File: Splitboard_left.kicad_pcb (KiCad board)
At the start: 2 copper layers, 124.1 x 95.1 mm, 63 parts, among them J1 USB_C_Receptacle_USB2.0, J2 TRRS, U1 ATmega32U4-AU, Y1 16MHz

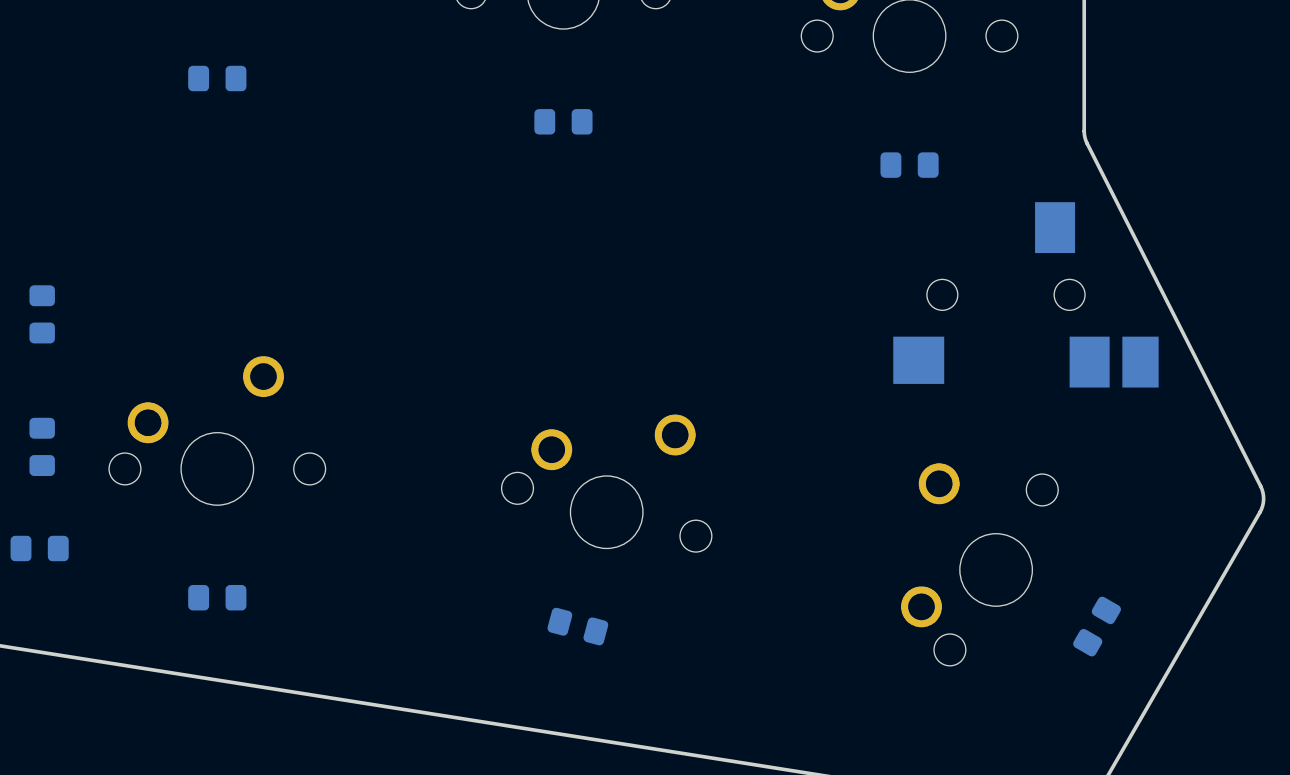
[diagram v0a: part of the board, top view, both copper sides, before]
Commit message: save
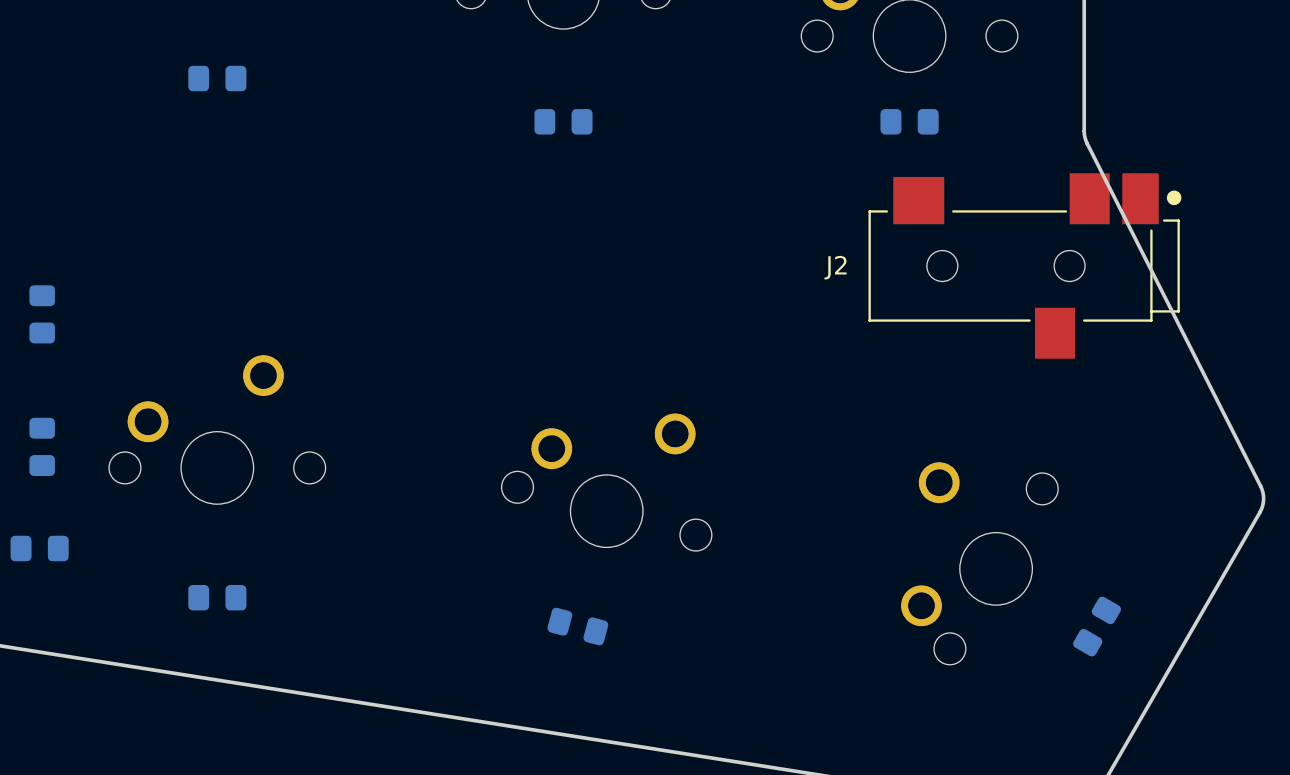
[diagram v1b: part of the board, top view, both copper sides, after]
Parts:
- J2: moved to F.Cu
- moved D52 2.38 mm to (176.9, 89.6)
- moved J2 1.59 mm to (182.5, 97.6)
- moved KC_53 0.06 mm to (181.7, 114.2)
- moved KC_43 0.06 mm to (160.3, 111.1)
- moved KC_33 0.06 mm to (138.8, 108.7)
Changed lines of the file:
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@@
   )
   (module MX_Only:MXOnly-1U-NoLED (layer F.Cu)
-    (at 181.673257 114.298749 60)
+    (at 181.673257 114.239952 60)
     (fp_text reference KC_53 (at 0 3.175 60) (layer Dwgs.User)
       (effects (font (size 1 1) (thickness 0.15)))
@@
   )
   (module MX_Only:MXOnly-1U-NoLED (layer F.Cu)
-    (at 160.253266 111.123749 345)
+    (at 160.253266 111.06662 345)
     (fp_text reference KC_43 (at 0 3.175 165) (layer Dwgs.User)
       (effects (font (size 1 1) (thickness 0.15)))
@@
   )
   (module MX_Only:MXOnly-1U-NoLED (layer F.Cu)
-    (at 138.833275 108.742499)
+    (at 138.833275 108.686621)
     (fp_text reference KC_33 (at 0 3.175) (layer Dwgs.User)
       (effects (font (size 1 1) (thickness 0.15)))
@@
     (pad "" np_thru_hole circle (at 5.08 0 48.0996) (size 1.75 1.75) (drill 1.75) (layers *.Cu *.Mask))
   )
-  (module SJ-43514-SMT:CUI_SJ-43514-SMT (layer B.Cu)
-    (at 182.46659 99.166625 180)
-    (fp_text reference J2 (at 9.519996 0) (layer B.SilkS)
-      (effects (font (size 1.004591 1.004591) (thickness 0.15)) (justify mirror))
-    )
-    (fp_text value TRRS (at 0.91336 -6.392105) (layer B.Fab)
-      (effects (font (size 1.003724 1.003724) (thickness 0.015)) (justify mirror))
-    )
-    (fp_line (start -9.5 -2.75) (end -9.5 2.75) (layer B.CrtYd) (width 0.05))
-    (fp_line (start -8.5 -2.75) (end -9.5 -2.75) (layer B.CrtYd) (width 0.05))
-    (fp_line (start -8.5 -5.5) (end -8.5 -2.75) (layer B.CrtYd) (width 0.05))
-    (fp_line (start -3 -5.5) (end -8.5 -5.5) (layer B.CrtYd) (width 0.05))
-    (fp_line (start -3 -3.25) (end -3 -5.5) (layer B.CrtYd) (width 0.05))
-    (fp_line (start 3.25 -3.25) (end -3 -3.25) (layer B.CrtYd) (width 0.05))
-    (fp_line (start 3.25 -5.5) (end 3.25 -3.25) (layer B.CrtYd) (width 0.05))
-    (fp_line (start 6.75 -5.5) (end 3.25 -5.5) (layer B.CrtYd) (width 0.05))
-    (fp_line (start 6.75 -3.25) (end 6.75 -5.5) (layer B.CrtYd) (width 0.05))
-    (fp_line (start 8 -3.25) (end 6.75 -3.25) (layer B.CrtYd) (width 0.05))
-    (fp_line (start 8 3.25) (end 8 -3.25) (layer B.CrtYd) (width 0.05))
-    (fp_line (start -1.1 3.25) (end 8 3.25) (layer B.CrtYd) (width 0.05))
-    (fp_line (start -1.1 5.35) (end -1.1 3.25) (layer B.CrtYd) (width 0.05))
-    (fp_line (start -3.8 5.35) (end -1.1 5.35) (layer B.CrtYd) (width 0.05))
-    (fp_line (start -3.8 3.25) (end -3.8 5.35) (layer B.CrtYd) (width 0.05))
-    (fp_line (start -8 3.25) (end -3.8 3.25) (layer B.CrtYd) (width 0.05))
-    (fp_line (start -8 2.75) (end -8 3.25) (layer B.CrtYd) (width 0.05))
-    (fp_line (start -9.5 2.75) (end -8 2.75) (layer B.CrtYd) (width 0.05))
-    (fp_line (start 7.75 3) (end 7.75 -3) (layer B.SilkS) (width 0.127))
-    (fp_circle (center -9 -3.75) (end -8.8 -3.75) (layer B.SilkS) (width 0.4))
-    (fp_line (start 7.75 3) (end -1.05 3) (layer B.SilkS) (width 0.127))
-    (fp_line (start 6.8 -3) (end 7.75 -3) (layer B.SilkS) (width 0.127))
-    (fp_line (start -3.05 -3) (end 3.15 -3) (layer B.SilkS) (width 0.127))
-    (fp_line (start -9.25 -2.5) (end -8.45 -2.5) (layer B.SilkS) (width 0.127))
-    (fp_line (start -9.25 2.5) (end -9.25 -2.5) (layer B.SilkS) (width 0.127))
-    (fp_line (start -7.75 2.5) (end -9.25 2.5) (layer B.SilkS) (width 0.127))
-    (fp_line (start -7.75 2.5) (end -7.75 -1.95) (layer B.SilkS) (width 0.127))
-    (fp_line (start -7.75 3) (end -7.75 2.5) (layer B.SilkS) (width 0.127))
-    (fp_line (start -4.05 3) (end -7.75 3) (layer B.SilkS) (width 0.127))
-    (fp_line (start -9.25 -2.5) (end -7.75 -2.5) (layer B.Fab) (width 0.127))
-    (fp_line (start -9.25 2.5) (end -9.25 -2.5) (layer B.Fab) (width 0.127))
-    (fp_line (start -7.75 2.5) (end -9.25 2.5) (layer B.Fab) (width 0.127))
-    (fp_line (start 7.75 3) (end -7.75 3) (layer B.Fab) (width 0.127))
-    (fp_line (start 7.75 -3) (end 7.75 3) (layer B.Fab) (width 0.127))
-    (fp_line (start -7.75 -3) (end 7.75 -3) (layer B.Fab) (width 0.127))
-    (fp_line (start -7.75 -2.5) (end -7.75 -3) (layer B.Fab) (width 0.127))
-    (fp_line (start -7.75 2.5) (end -7.75 -2.5) (layer B.Fab) (width 0.127))
-    (fp_line (start -7.75 3) (end -7.75 2.5) (layer B.Fab) (width 0.127))
+  (module SJ-43514-SMT:CUI_SJ-43514-SMT (layer F.Cu)
+    (at 182.46659 97.579959 180)
+    (fp_text reference J2 (at 9.519996 0) (layer F.SilkS)
+      (effects (font (size 1.004591 1.004591) (thickness 0.15)))
+    )
+    (fp_text value TRRS (at 0.91336 6.392105) (layer F.Fab)
+      (effects (font (size 1.003724 1.003724) (thickness 0.015)))
+    )
+    (fp_line (start -9.5 2.75) (end -9.5 -2.75) (layer F.CrtYd) (width 0.05))
+    (fp_line (start -8.5 2.75) (end -9.5 2.75) (layer F.CrtYd) (width 0.05))
+    (fp_line (start -8.5 5.5) (end -8.5 2.75) (layer F.CrtYd) (width 0.05))
+    (fp_line (start -3 5.5) (end -8.5 5.5) (layer F.CrtYd) (width 0.05))
+    (fp_line (start -3 3.25) (end -3 5.5) (layer F.CrtYd) (width 0.05))
+    (fp_line (start 3.25 3.25) (end -3 3.25) (layer F.CrtYd) (width 0.05))
+    (fp_line (start 3.25 5.5) (end 3.25 3.25) (layer F.CrtYd) (width 0.05))
+    (fp_line (start 6.75 5.5) (end 3.25 5.5) (layer F.CrtYd) (width 0.05))
+    (fp_line (start 6.75 3.25) (end 6.75 5.5) (layer F.CrtYd) (width 0.05))
+    (fp_line (start 8 3.25) (end 6.75 3.25) (layer F.CrtYd) (width 0.05))
+    (fp_line (start 8 -3.25) (end 8 3.25) (layer F.CrtYd) (width 0.05))
+    (fp_line (start -1.1 -3.25) (end 8 -3.25) (layer F.CrtYd) (width 0.05))
+    (fp_line (start -1.1 -5.35) (end -1.1 -3.25) (layer F.CrtYd) (width 0.05))
+    (fp_line (start -3.8 -5.35) (end -1.1 -5.35) (layer F.CrtYd) (width 0.05))
+    (fp_line (start -3.8 -3.25) (end -3.8 -5.35) (layer F.CrtYd) (width 0.05))
+    (fp_line (start -8 -3.25) (end -3.8 -3.25) (layer F.CrtYd) (width 0.05))
+    (fp_line (start -8 -2.75) (end -8 -3.25) (layer F.CrtYd) (width 0.05))
+    (fp_line (start -9.5 -2.75) (end -8 -2.75) (layer F.CrtYd) (width 0.05))
+    (fp_line (start 7.75 -3) (end 7.75 3) (layer F.SilkS) (width 0.127))
+    (fp_circle (center -9 3.75) (end -8.8 3.75) (layer F.SilkS) (width 0.4))
+    (fp_line (start 7.75 -3) (end -1.05 -3) (layer F.SilkS) (width 0.127))
+    (fp_line (start 6.8 3) (end 7.75 3) (layer F.SilkS) (width 0.127))
+    (fp_line (start -3.05 3) (end 3.15 3) (layer F.SilkS) (width 0.127))
+    (fp_line (start -9.25 2.5) (end -8.45 2.5) (layer F.SilkS) (width 0.127))
+    (fp_line (start -9.25 -2.5) (end -9.25 2.5) (layer F.SilkS) (width 0.127))
+    (fp_line (start -7.75 -2.5) (end -9.25 -2.5) (layer F.SilkS) (width 0.127))
+    (fp_line (start -7.75 -2.5) (end -7.75 1.95) (layer F.SilkS) (width 0.127))
+    (fp_line (start -7.75 -3) (end -7.75 -2.5) (layer F.SilkS) (width 0.127))
+    (fp_line (start -4.05 -3) (end -7.75 -3) (layer F.SilkS) (width 0.127))
+    (fp_line (start -9.25 2.5) (end -7.75 2.5) (layer F.Fab) (width 0.127))
+    (fp_line (start -9.25 -2.5) (end -9.25 2.5) (layer F.Fab) (width 0.127))
+    (fp_line (start -7.75 -2.5) (end -9.25 -2.5) (layer F.Fab) (width 0.127))
+    (fp_line (start 7.75 -3) (end -7.75 -3) (layer F.Fab) (width 0.127))
+    (fp_line (start 7.75 3) (end 7.75 -3) (layer F.Fab) (width 0.127))
+    (fp_line (start -7.75 3) (end 7.75 3) (layer F.Fab) (width 0.127))
+    (fp_line (start -7.75 2.5) (end -7.75 3) (layer F.Fab) (width 0.127))
+    (fp_line (start -7.75 -2.5) (end -7.75 2.5) (layer F.Fab) (width 0.127))
+    (fp_line (start -7.75 -3) (end -7.75 -2.5) (layer F.Fab) (width 0.127))
     (pad None np_thru_hole circle (at 3.75 0 180) (size 1.7 1.7) (drill 1.7) (layers *.Cu *.Mask))
     (pad None np_thru_hole circle (at -3.25 0 180) (size 1.7 1.7) (drill 1.7) (layers *.Cu *.Mask))
-    (pad 4 smd rect (at -4.35 -3.7 180) (size 2.2 2.8) (layers B.Cu B.Paste B.Mask)
+    (pad 4 smd rect (at -4.35 3.7 180) (size 2.2 2.8) (layers F.Cu F.Paste F.Mask)
       (net 37 SCL))
-    (pad 3 smd rect (at -2.45 3.7 180) (size 2.2 2.8) (layers B.Cu B.Paste B.Mask)
+    (pad 3 smd rect (at -2.45 -3.7 180) (size 2.2 2.8) (layers F.Cu F.Paste F.Mask)
       (net 38 SDA))
-    (pad 2 smd rect (at 5.05 -3.6 180) (size 2.8 2.6) (layers B.Cu B.Paste B.Mask)
-      (net 1 GND))
-    (pad 1 smd rect (at -7.15 -3.7 180) (size 2 2.8) (layers B.Cu B.Paste B.Mask)
+    (pad 2 smd rect (at 5.05 3.6 180) (size 2.8 2.6) (layers F.Cu F.Paste F.Mask)
+      (net 1 GND))
+    (pad 1 smd rect (at -7.15 3.7 180) (size 2 2.8) (layers F.Cu F.Paste F.Mask)
       (net 2 +5V))
   )
@@
   )
   (module Diode_SMD:D_0805_2012Metric_Pad1.15x1.40mm_HandSolder (layer B.Cu)
-    (at 176.913259 92.026628)
+    (at 176.913259 89.646629)
     (descr "Diode SMD 0805 (2012 Metric), square (rectangular) end terminal, IPC_7351 nominal, (Body size source: https://docs.google.com/spreadsheets/d/1BsfQQcO9C6DZCsRaXUlFlo91Tg2WpOkGARC1WS5S8t0/edit?usp=sharing), generated with kicad-footprint-generator")
     (tags "diode handsolder")
